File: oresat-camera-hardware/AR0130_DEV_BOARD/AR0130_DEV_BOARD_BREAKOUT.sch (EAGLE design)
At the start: 2 parts, among them J1 4-1734592-0

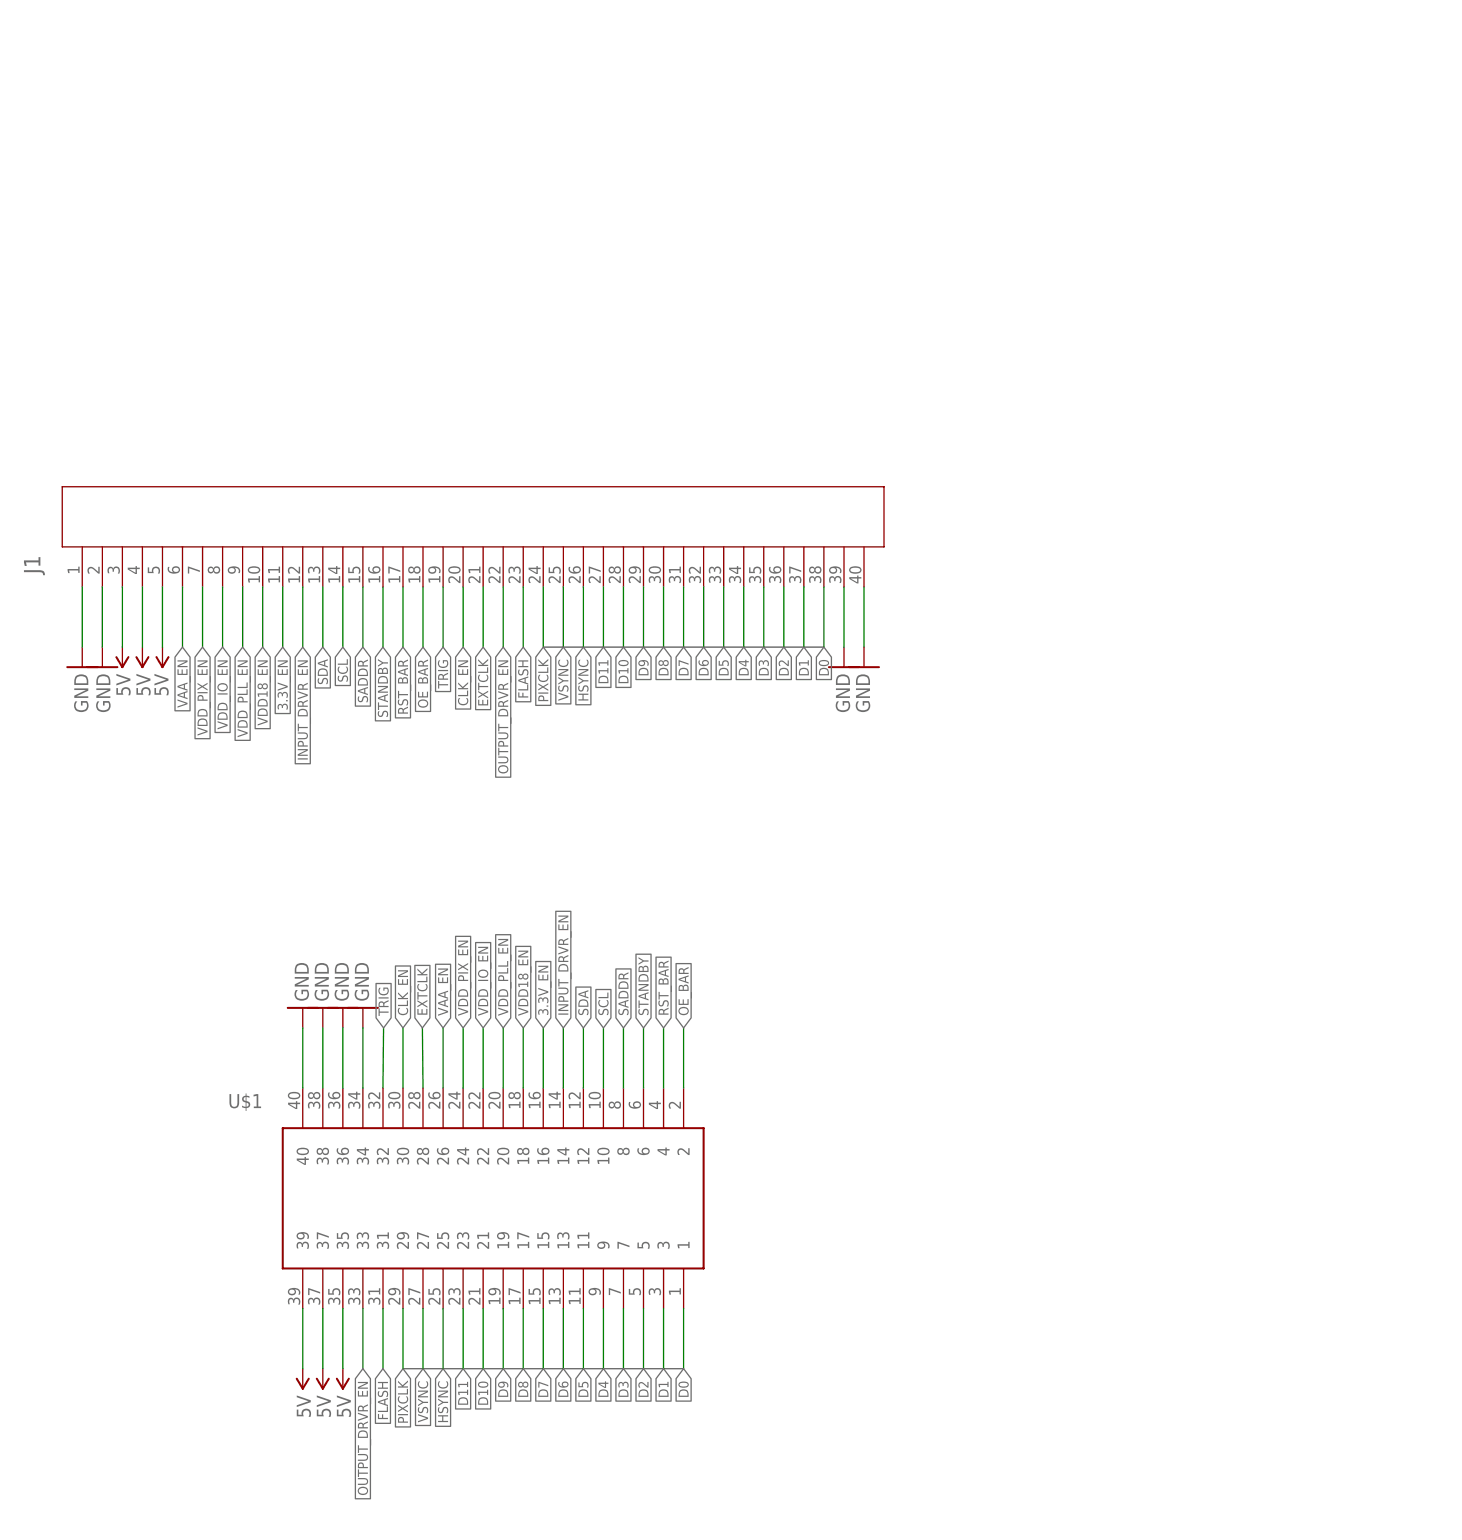
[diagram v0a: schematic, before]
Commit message: finishing touches!
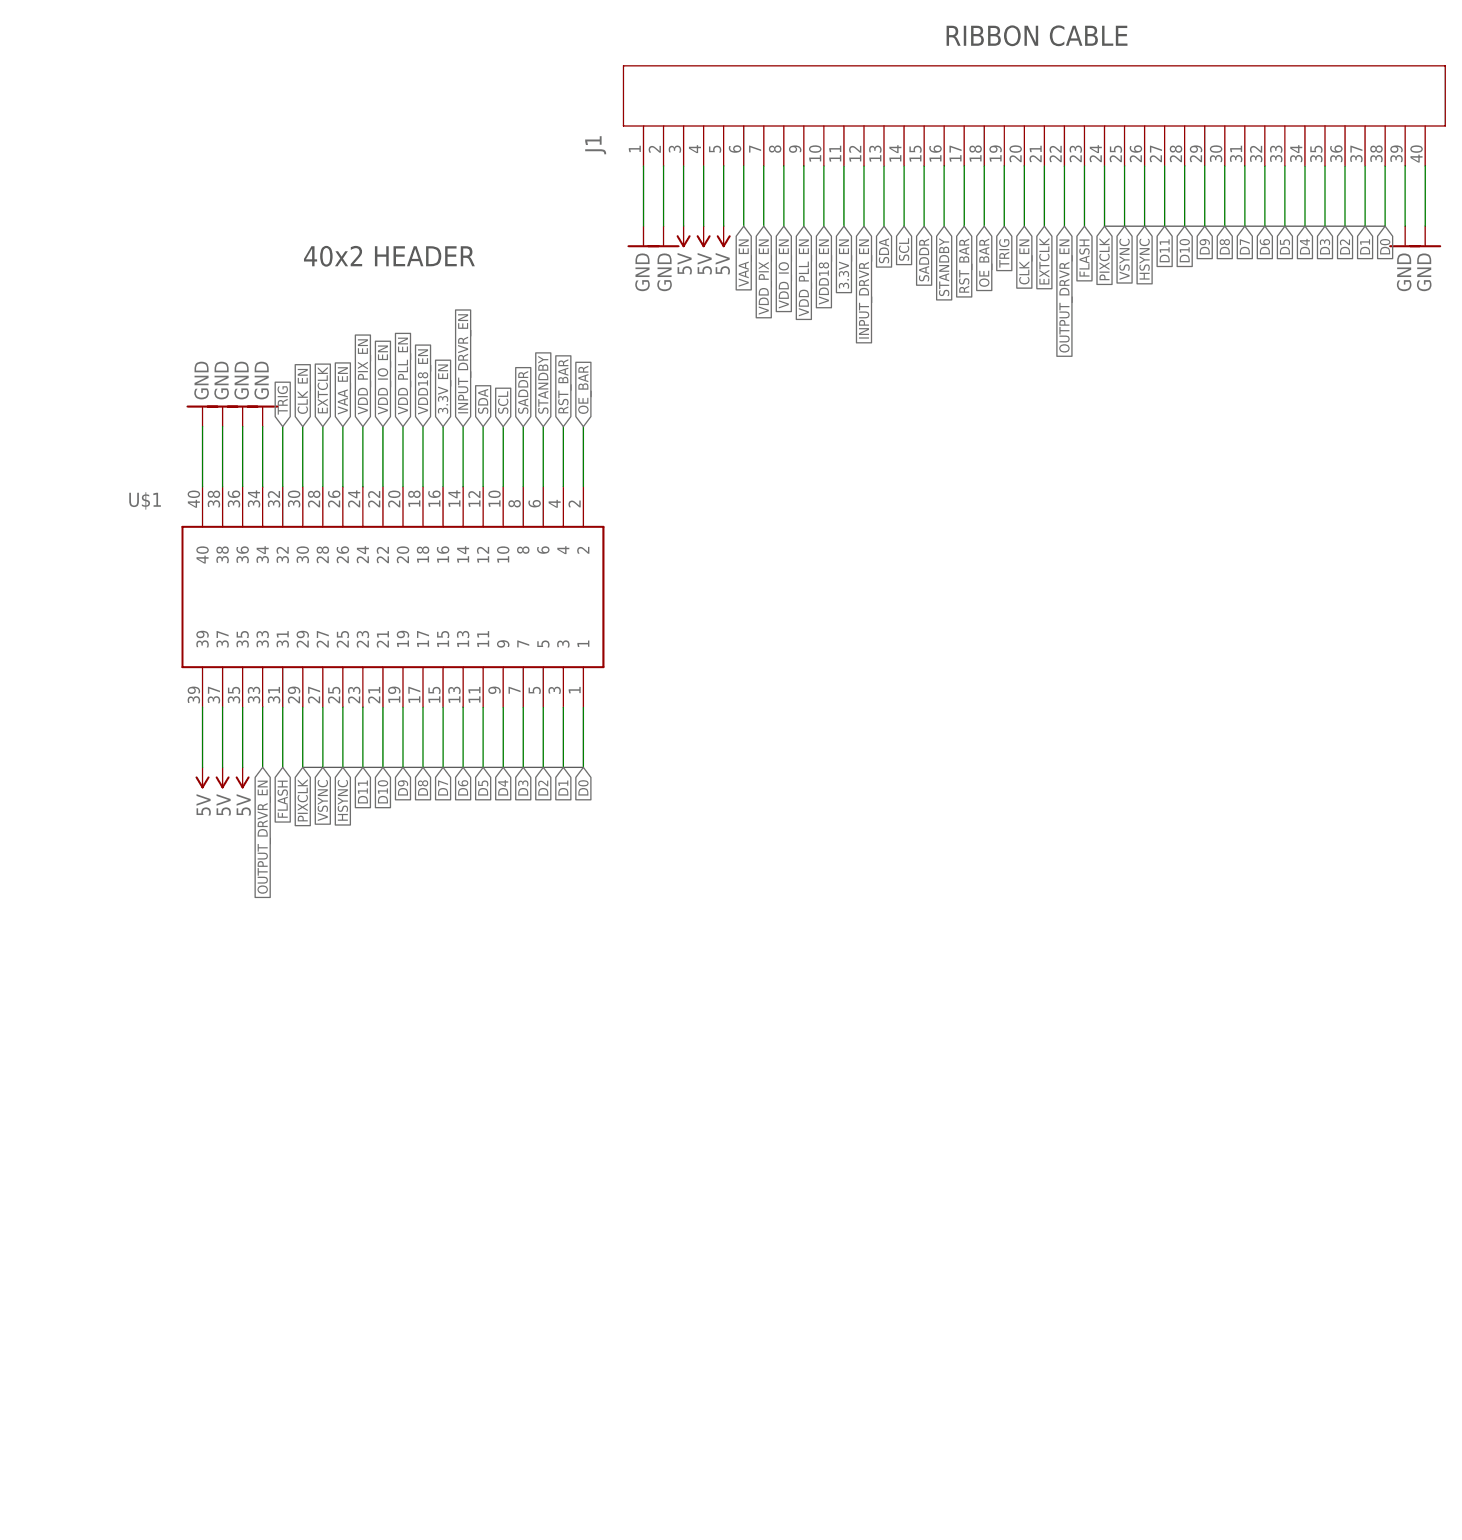
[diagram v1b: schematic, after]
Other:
- note added: "40x2 HEADER"
- note added: "RIBBON CABLE"
- moved on the sheet: J1, U$1
